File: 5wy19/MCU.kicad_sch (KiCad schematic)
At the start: 25 parts, among them IC1 C167, Y1 Crystal

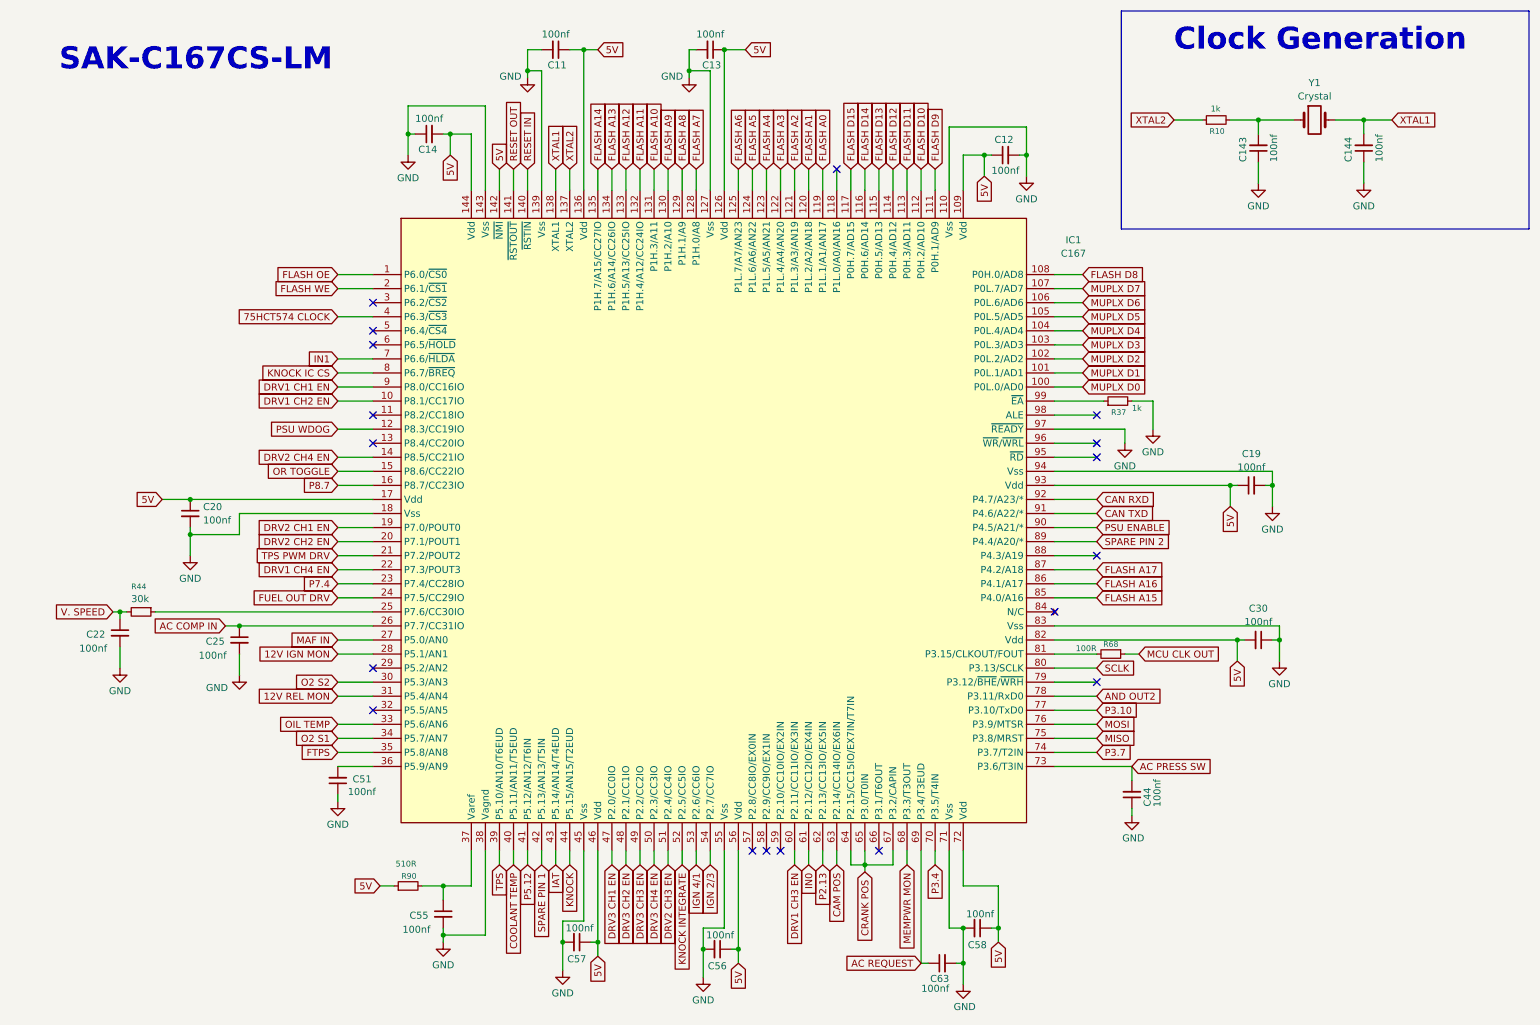
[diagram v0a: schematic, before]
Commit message: Final schematic (except maybe some oversights)
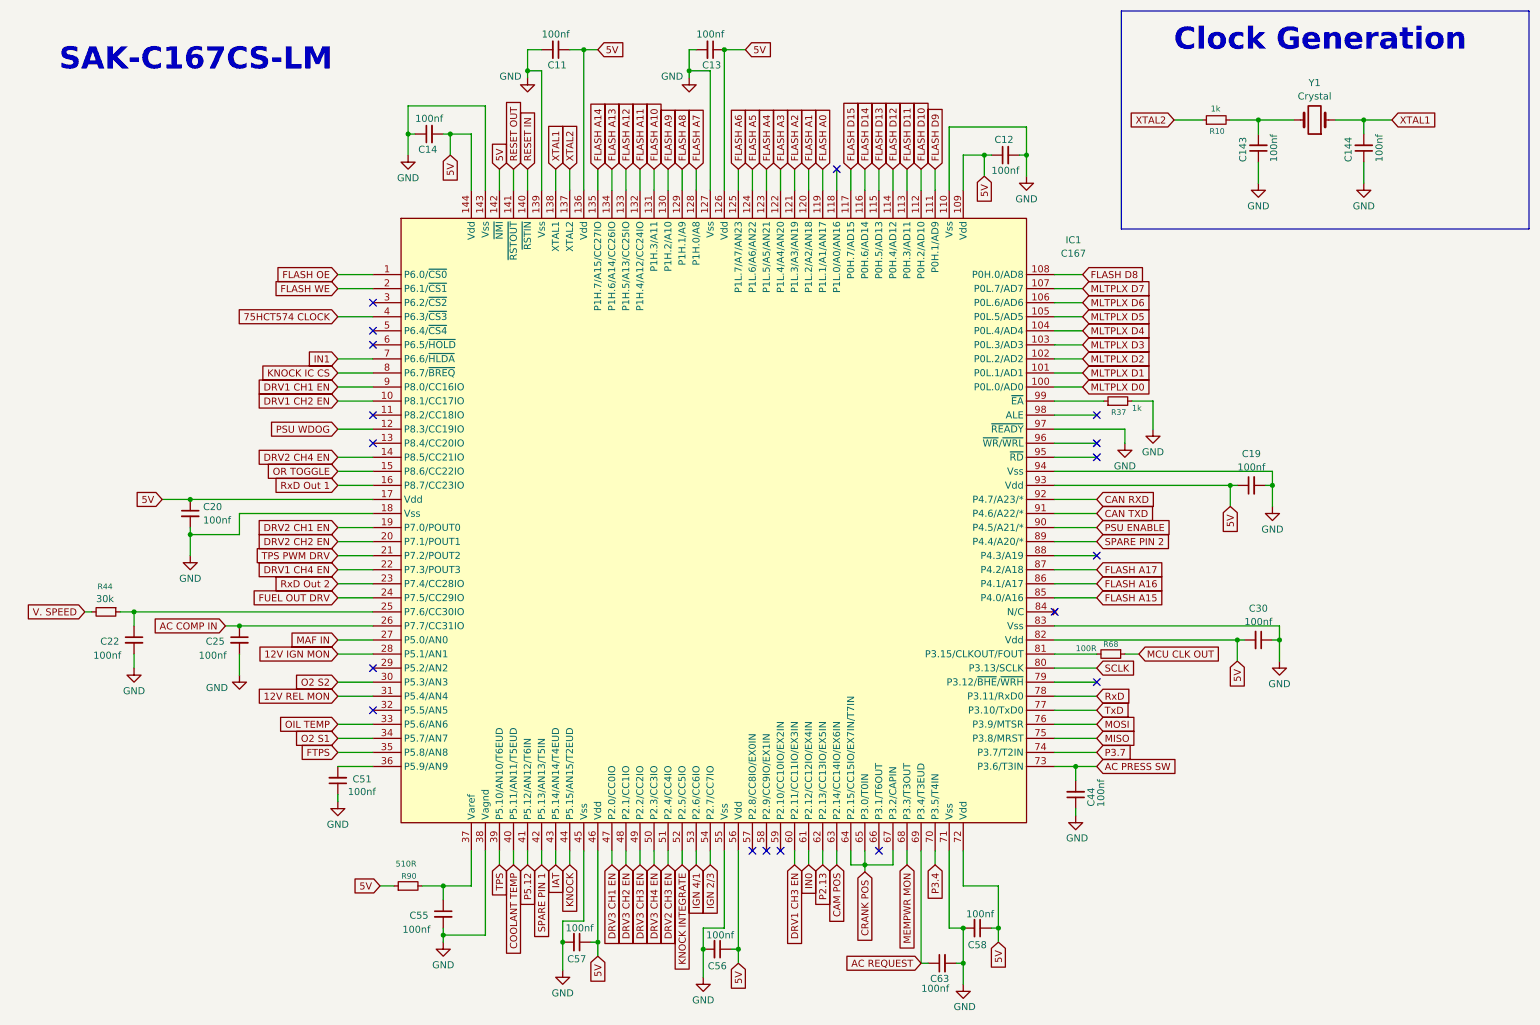
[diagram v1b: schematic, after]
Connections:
- net V. SPEED: no longer C22.1
- net XTAL1: now also Y1.1; no longer Y1.2
- net at C143.2, R10.2: now also Y1.2; no longer Y1.1
- net at IC1.25 (P7.6/CC30IO), R44.1: now also C22.1
- net AND OUT2 renamed RxD
- net MUPLX D0 renamed MLTPLX D0
- net MUPLX D1 renamed MLTPLX D1
- net MUPLX D2 renamed MLTPLX D2
- net MUPLX D3 renamed MLTPLX D3
- net MUPLX D4 renamed MLTPLX D4
- net MUPLX D5 renamed MLTPLX D5
- net MUPLX D6 renamed MLTPLX D6
- net MUPLX D7 renamed MLTPLX D7
- net P3.10 renamed TxD
- net P7.4 renamed RxD Out 2
- net P8.7 renamed RxD Out 1
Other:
- moved on the sheet: C22, C44, R44, Y1
